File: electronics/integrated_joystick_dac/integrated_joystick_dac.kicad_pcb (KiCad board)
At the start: 2 copper layers, 53.3 x 52.1 mm, 13 parts, among them J1 Power/Signal Out, U1 raspberry_pi_pico, U2 MCP4728

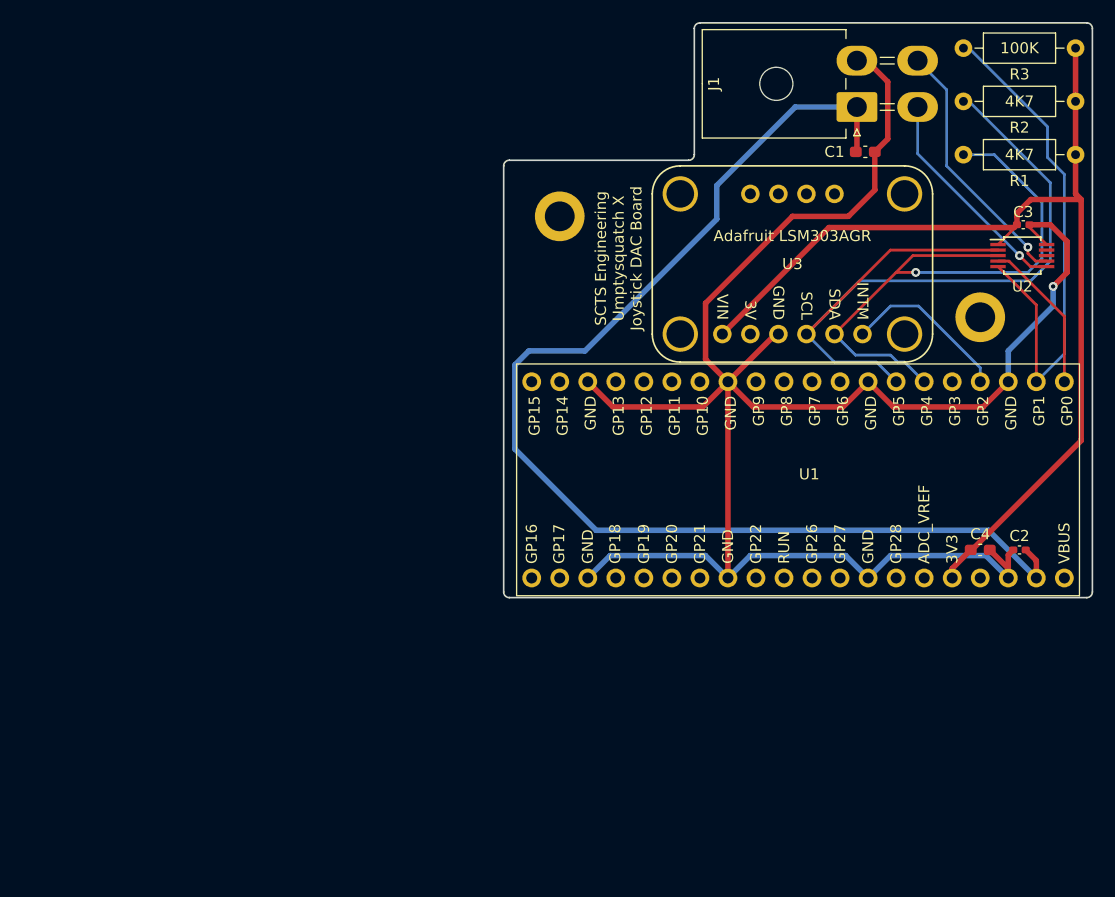
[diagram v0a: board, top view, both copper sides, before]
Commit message: modify pcb and schematic sheets for export for design report
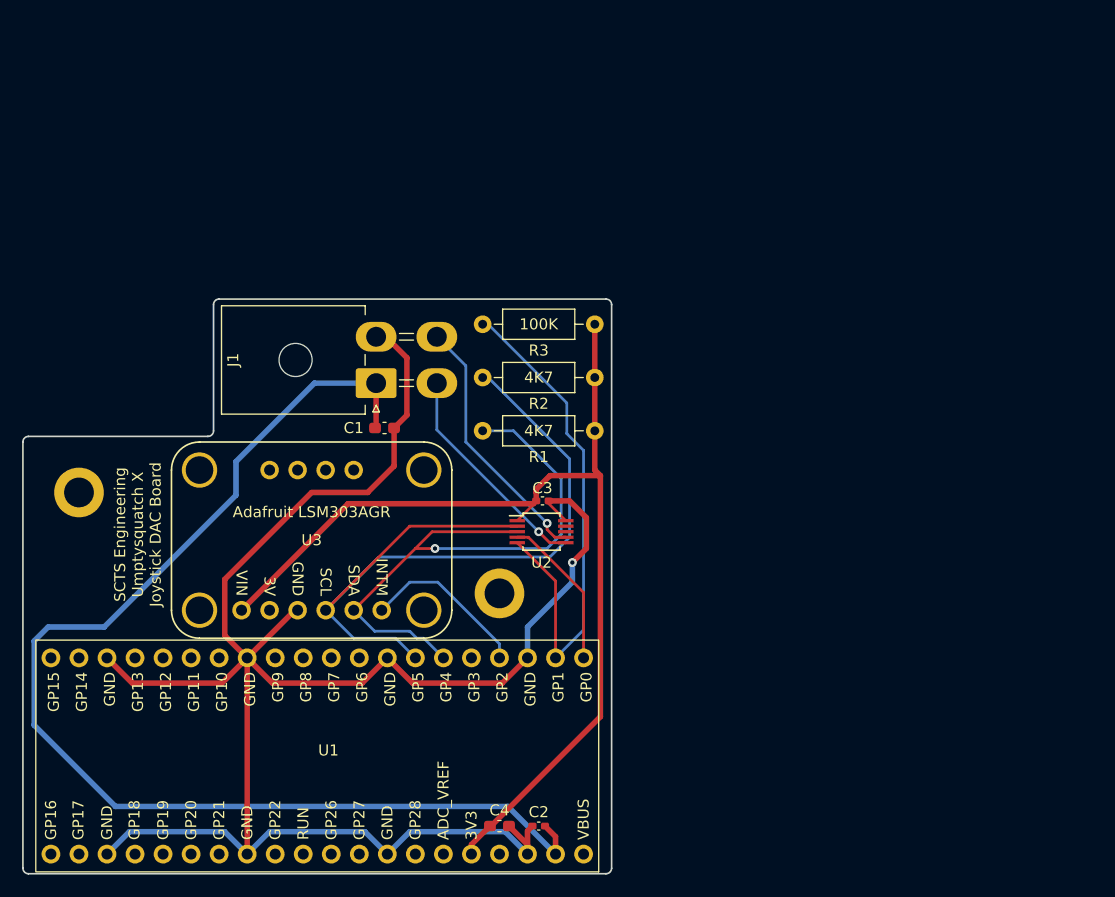
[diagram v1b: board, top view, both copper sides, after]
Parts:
- moved C4 50.2 mm to (153.8, 124.6)
- moved R2 50.2 mm to (162.4, 83.9)
- moved REF** 50.2 mm to (115.7, 94.4)
- moved U1 50.2 mm to (138.5, 117.9)
- moved U2 50.2 mm to (157.6, 97.9)
- moved U3 50.2 mm to (136.8, 98.7)
- moved R1 50.2 mm to (162.4, 88.8)
- moved R3 50.2 mm to (162.4, 79.1)
- moved REF** 50.2 mm to (153.8, 103.5)
- moved C1 50.2 mm to (143.4, 88.5)
- moved C2 50.2 mm to (157.4, 124.6)
- moved C3 50.2 mm to (157.7, 95.1)
- moved J1 50.2 mm to (142.6, 84.5)
